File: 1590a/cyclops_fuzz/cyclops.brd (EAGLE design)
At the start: 33 x 52.1 mm, 44 parts, among them IC1 4558, IC2 741

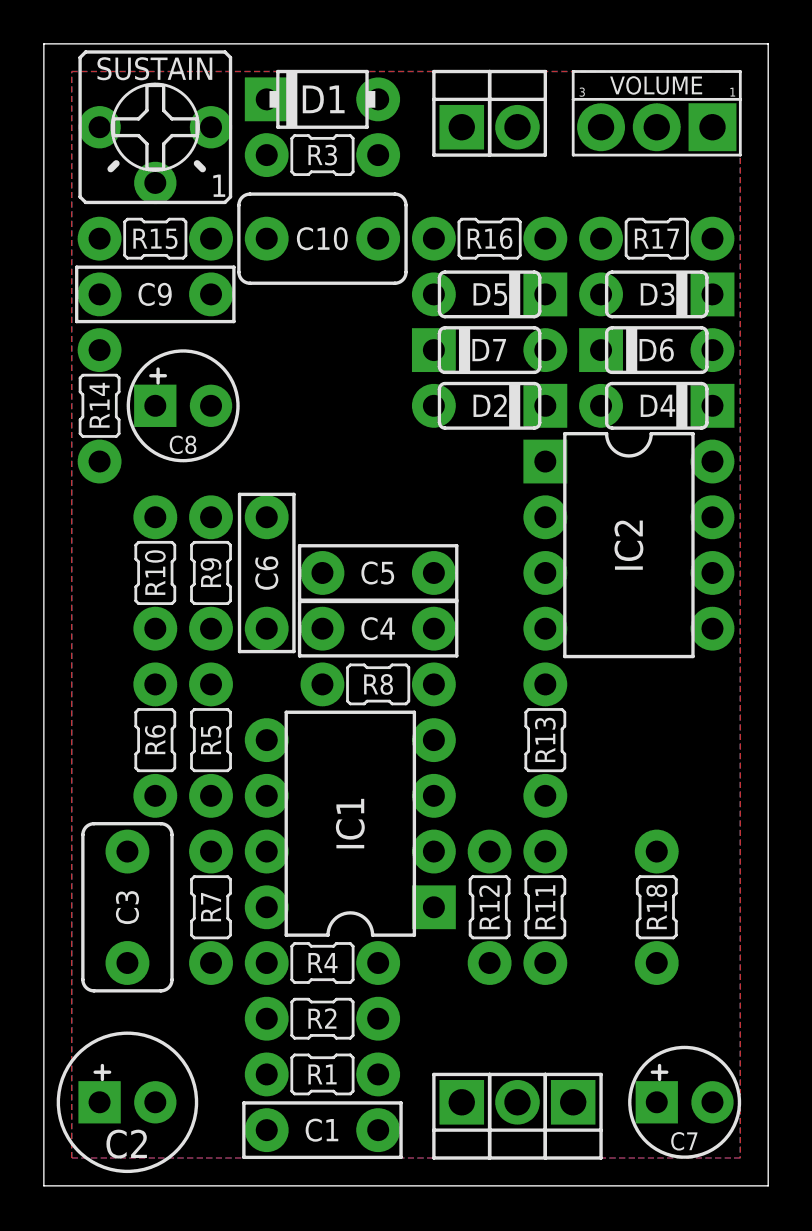
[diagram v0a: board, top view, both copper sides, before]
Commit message: updates to cerberus and cyclops
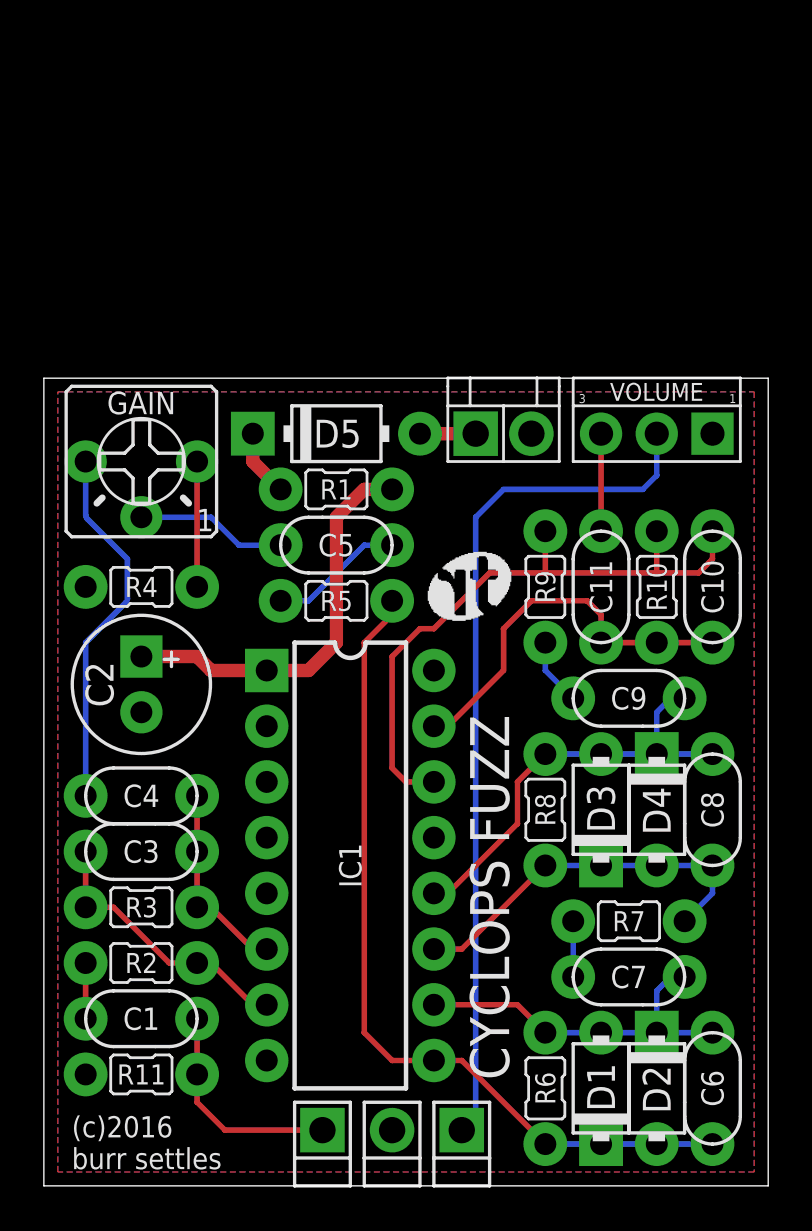
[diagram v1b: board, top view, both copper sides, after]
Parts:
- removed D6, D7: 1N914, diodes:DO35-2
- removed IC2: 741, integrated circuits:DIL08
- removed PAD1, PAD2, PAD5: PADSQR, supply pins:SQUARE
- removed PAD3, PAD4: PADRND, supply pins:ROUND
- removed R12: 560k, resistors:R0207/2V
- removed R13: 47R, resistors:R0207/2V
- removed R14: 8k2, resistors:R0207/2V
- removed R15: 470k, resistors:R0207/2V
- removed R16, R17: 47k, resistors:R0207/2V
- removed R18: 100k, resistors:R0207/2V
- removed SUSTAIN: 10kB, potentiometers:2262_TRIM
- added 9V: DC_MONO, jacks:DC
- added C11: 100n, capacitors-film:050X030_025_2
- added GAIN: 100kA, potentiometers:2262_TRIM
- added GND: PADRND, supply pins:ROUND
- added IN, OUT: PADSQR, supply pins:SQUARE
- added U$1: (no value), logos:RT150
- C1: value 150nF -> 47n; device capacitors-film:BOX_SMALL -> capacitors-film:050X030_025_2
- C10: value 1uF -> 150p; device capacitors-film:BOX_MED -> capacitors-film:050X030_025_2
- C3: value 1uF -> 220p; device capacitors-film:BOX_MED -> capacitors-film:050X030_025_2
- C4: value 10nF -> 100n; device capacitors-film:BOX_SMALL -> capacitors-film:050X030_025_2
- C5: value 4.7nF -> 100n; device capacitors-film:BOX_SMALL -> capacitors-film:050X030_025_2
- C6: value .22uF -> 150p; device capacitors-film:BOX_SMALL -> capacitors-film:050X030_025_2
- C7: value 10uF -> 100n; device capacitors-elec:050_020_1 -> capacitors-film:050X030_025_2
- C8: value 1uF -> 150p; device capacitors-elec:050_020_1 -> capacitors-film:050X030_025_2
- C9: value 150pF -> 100n; device capacitors-film:BOX_SMALL -> capacitors-film:050X030_025_2
- D1: value 1N5817 -> (none)
- D2, D3, D4: value 1N914 -> (none); device diodes:DO35-2 -> diodes:DO41-2
- D5: value 1N914 -> 1N5417; device diodes:DO35-2 -> diodes:DO41-3
- IC1: value 4558 -> CD4049; device integrated circuits:DIL08 -> integrated circuits:DIL16
- R1, R9: value 1M -> 100k
- R10: value 820k -> 330k
- R11: value 62k -> 1M
- R2: value 56k -> 100k
- R3: value 47R -> 1M
- R4: value 330k -> 1k
- R5: value 220k -> 33k
- R6: value 220k -> 1M
- R7: value 10k -> 33k
- R8: value 47k -> 1M
- moved D1 46.8 mm to (25.4, 4.45), turned to 90 degrees
- moved R3 35.3 mm to (4.45, 12.7)
- moved D2 32.0 mm to (27.9, 4.45), turned to 270 degrees
- moved C6 31.1 mm to (30.5, 4.45)
- moved C8 30.4 mm to (30.5, 17.1), turned to 270 degrees
- moved C9 28.4 mm to (26.7, 22.2)
- moved R1 26.7 mm to (13.3, 31.8)
- moved C10 23.8 mm to (30.5, 27.3), turned to 90 degrees
- moved R6 23.8 mm to (22.9, 4.45)
- moved D3 23.6 mm to (25.4, 17.1), turned to 90 degrees
- moved R10 22.9 mm to (27.9, 27.3)
- moved R11 19.9 mm to (4.45, 5.08), turned to 0 degrees
- moved C2 19.1 mm to (4.45, 22.9), turned to 270 degrees
- moved R7 19.1 mm to (26.7, 12.1), turned to 0 degrees
- moved R4 19.0 mm to (4.45, 27.3), turned to 0 degrees
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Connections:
- removed net +9V: D1.A, PAD1.1
- removed net N$19: D5.A, D7.C
- removed net N$20: D3.A, D5.C
- removed net VA: C2.+, IC1.8, IC2.7, R10.2, R3.2, R6.2
- removed net VB: C3.1, IC1.5, R5.2, R6.1
- removed net VC: C6.1, IC2.3, R10.1, R9.2
- new net N$15: GAIN.1, R4.2
- net GND: now also 9V.S, GND.1, IC1.3, IC1.5, IC1.8, R11.1, R4.1; no longer C3.2, C4.2, C6.2, C7.-, IC1.4, IC2.4, PAD3.1, PAD4.1, R1.1, R17.1, R18.1, R5.1, R9.1
- net IN: now also C1.2, IN.1, R11.2; no longer C1.1, PAD2.1, R1.2
- net N$1: now also C3.1, C4.2, IC1.6, R3.2; no longer C1.2, R2.1
- net N$10: now also C4.1, GAIN.3; no longer C7.+, R11.1, R13.1
- net N$11: now also C8.1, C9.2, D3.A, D4.C, IC1.12, R8.2; no longer R13.2, SUSTAIN.1
- net N$12: now also C9.1, R9.1; no longer D1.C, R3.1
- net N$13: now also C10.2, IC1.14, R10.1, R9.2; no longer C8.-, SUSTAIN.2
- net N$14: now also C10.1, C11.2, IC1.15, R10.2; no longer C8.+, R14.1
- net N$16: now also C11.1, VOLUME.3; no longer C9.1, D2.A, D3.C, IC2.2, R14.2, R15.1
- net N$17: now also 9V.T, D5.A; no longer D2.C, D4.A
- net N$18: now also C2.+, IC1.1, R1.2; no longer D4.C, D6.A
- net N$2: now also C5.2, GAIN.2; no longer C10.2, R16.1
- net N$21: now also D5.C, R1.1; no longer C10.1, C9.2, D6.C, D7.A, IC2.6, R15.2
- net N$3: now also C3.2, IC1.7, R2.2, R3.1; no longer R16.2, R17.2, VOLUME.3
- net N$4: now also C1.1, R2.1; no longer IC1.6, R2.2, R4.1
- net N$5: now also C5.1, R5.1; no longer IC1.7, R4.2, R7.1
- net N$6: now also C6.2, D1.C, D2.A, IC1.9, R5.2, R6.1; no longer C5.1, R7.2, R8.1
- net N$7: now also C6.1, C7.2, D1.A, D2.C, IC1.10, R6.2; no longer C4.1, IC1.3, R8.2
- net N$8: now also C7.1, R7.1; no longer C5.2, IC1.1, R12.2, SUSTAIN.3
- net N$9: now also C8.2, D3.C, D4.A, IC1.11, R7.2, R8.1; no longer IC1.2, R11.2, R12.1
- net OUT: now also OUT.1; no longer PAD5.1, R18.2
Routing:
- net OUT: track 0.00 -> 39.1 mm
- net N$6: track 0.00 -> 38.2 mm
- net N$13: track 0.00 -> 28.8 mm
- net N$11: track 0.00 -> 19.9 mm
- net N$18: track 0.00 -> 18.5 mm
- net N$14: track 0.00 -> 17.7 mm
- net N$9: track 0.00 -> 17.3 mm
- net N$10: track 0.00 -> 16.8 mm
- net N$7: track 0.00 -> 16.7 mm
- net N$3: track 0.00 -> 12.6 mm
- net IN: track 0.00 -> 10.1 mm
- net N$1: track 0.00 -> 9.04 mm
- net N$2: track 0.00 -> 6.88 mm
- net N$5: track 0.00 -> 6.13 mm
- net N$15: track 0.00 -> 5.72 mm
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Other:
- board size 33 x 52.1 mm -> 33 x 36.8 mm
- board text added: "(c)2016 burr settles"
- board text added: "CYCLOPS FUZZ"
